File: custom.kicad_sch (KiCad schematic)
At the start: 43 parts, among them J1 OLED_128x32, SW1 Switch, U1 Nice_Nano_V2

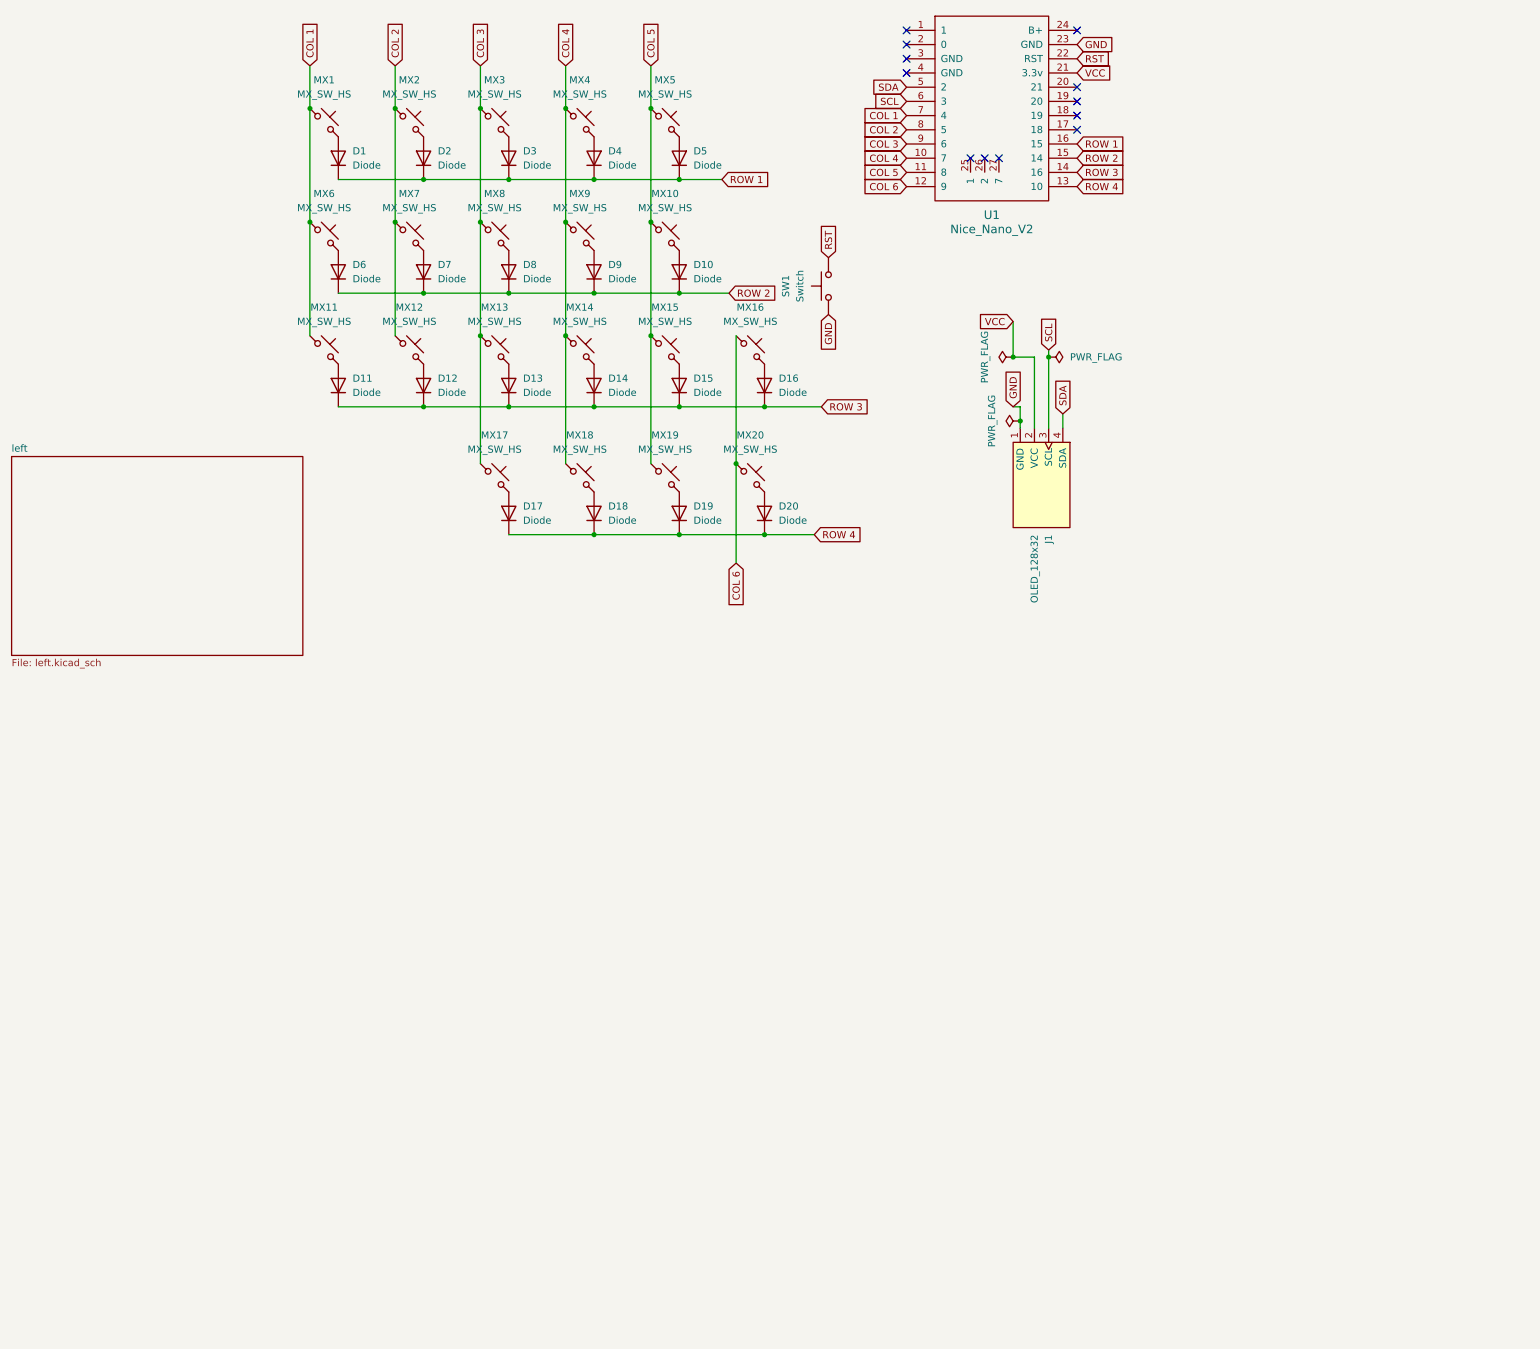
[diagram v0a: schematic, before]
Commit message: Formato de teclado listo
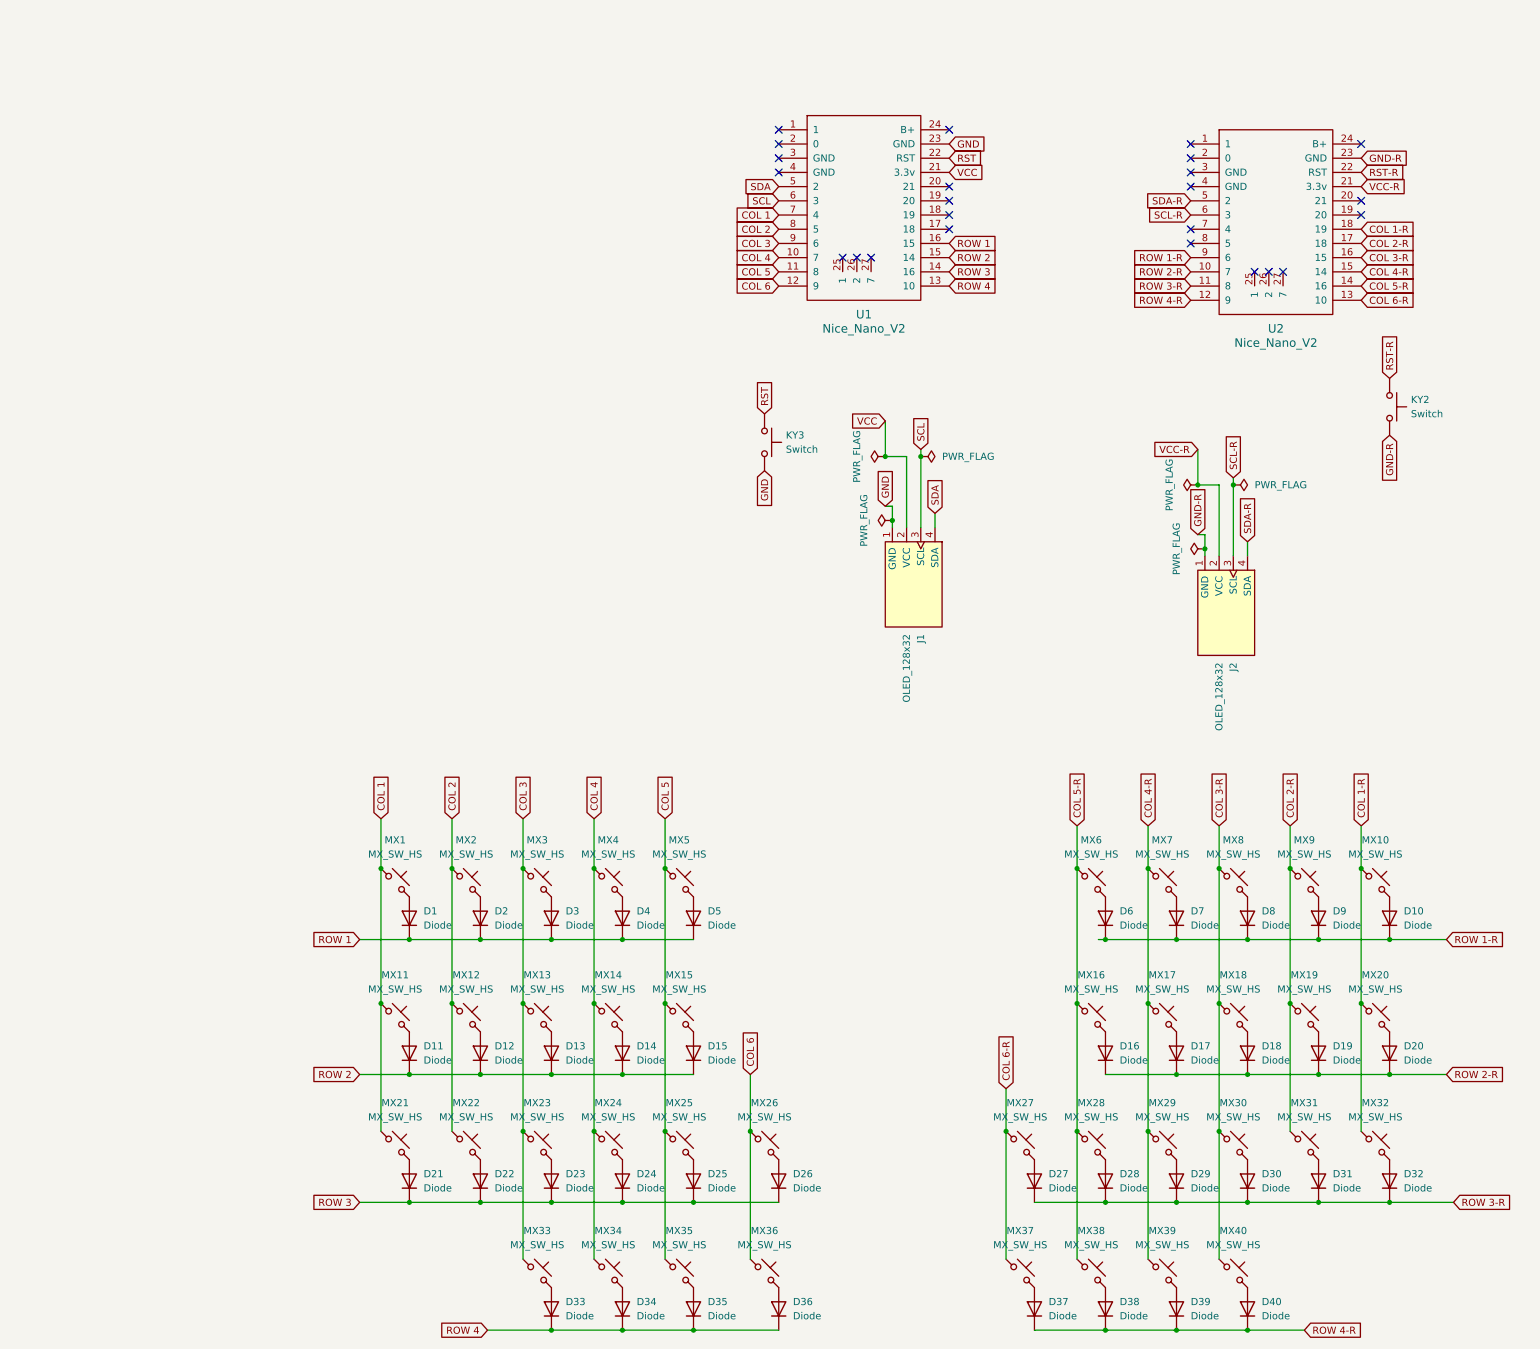
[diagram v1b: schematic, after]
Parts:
- removed SW1: Switch, Button_Switch_SMD:SW_Push_1P1T_NO_Vertical_Wuerth_434133025816, symbol ScottoKeebs:Placeholder_Switch
- added D21, D22, D23, D24, D25, D26, D27, D28, D29, D30, D31, D32, D33, D34, D35, D36, D37, D38, D39, D40: Diode, symbol ScottoKeebs:Placeholder_Diode
- added J2: OLED_128x32, ScottoKeebs_Components:OLED_128x32, symbol ScottoKeebs:OLED_128x32
- added KY2, KY3: Switch, Button_Switch_SMD:SW_Push_1P1T_NO_Vertical_Wuerth_434133025816, symbol ScottoKeebs:Placeholder_Switch
- added MX21, MX22, MX23, MX24, MX25, MX26, MX27, MX28, MX29, MX30, MX31, MX32, MX33, MX34, MX35, MX38, MX39, MX40: MX_SW_HS, PCM_marbastlib-mx:SW_MX_HS_CPG151101S11_1u, symbol PCM_marbastlib-mx:MX_SW_HS_CPG151101S11
- added MX36, MX37: MX_SW_HS, PCM_marbastlib-mx:SW_MX_HS_CPG151101S11_1.25u, symbol PCM_marbastlib-mx:MX_SW_HS_CPG151101S11
- added U2: Nice_Nano_V2, ScottoKeebs_MCU:Nice_Nano_V2, symbol ScottoKeebs:MCU_Nice_Nano_V2
- D1, D10, D11, D12, D13, D14, D15, D16, D17, D18, D19, D2, D20, D3, D4, D5, D6, D7, D8, D9: footprint Diode_SMD:D_SOD-123 -> (none)
- MX20: footprint PCM_marbastlib-mx:SW_MX_HS_CPG151101S11_1.25u -> PCM_marbastlib-mx:SW_MX_HS_CPG151101S11_1u
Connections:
- net COL 1: now also MX21.1; no longer MX6.1
- net COL 2: now also MX22.1; no longer MX7.1
- net COL 3: now also MX23.1, MX33.1; no longer MX17.1, MX8.1
- net COL 4: now also MX24.1, MX34.1; no longer MX18.1, MX9.1
- net COL 5: now also MX25.1, MX35.1; no longer MX10.1, MX19.1
- net COL 6: now also MX26.1, MX36.1; no longer MX16.1, MX20.1
- net GND: now also KY3.1
- net ROW 2: now also D11.1 (K), D12.1 (K), D13.1 (K), D14.1 (K), D15.1 (K); no longer D10.1 (K), D6.1 (K), D7.1 (K), D8.1 (K), D9.1 (K)
- net ROW 3: now also D21.1 (K), D22.1 (K), D23.1 (K), D24.1 (K), D25.1 (K), D26.1 (K); no longer D11.1 (K), D12.1 (K), D13.1 (K), D14.1 (K), D15.1 (K), D16.1 (K)
- net ROW 4: now also D33.1 (K), D34.1 (K), D35.1 (K), D36.1 (K); no longer D17.1 (K), D18.1 (K), D19.1 (K), D20.1 (K)
- net RST: now also KY3.2
- new net: D35.2 (A), MX35.2
- new net: D29.2 (A), MX29.2
- new net: D21.2 (A), MX21.2
- new net: D24.2 (A), MX24.2
- new net: D38.2 (A), MX38.2
- new net: D28.2 (A), MX28.2
- new net: D22.2 (A), MX22.2
- new net: D30.2 (A), MX30.2
- new net: D27.2 (A), MX27.2
- new net: D26.2 (A), MX26.2
- new net: D23.2 (A), MX23.2
- new net: D39.2 (A), MX39.2
- new net: D34.2 (A), MX34.2
- new net: D31.2 (A), MX31.2
- new net: D25.2 (A), MX25.2
- new net: D36.2 (A), MX36.2
- new net: D40.2 (A), MX40.2
- new net: D33.2 (A), MX33.2
- new net: D32.2 (A), MX32.2
- new net: D37.2 (A), MX37.2
- new net COL 1-R: MX10.1, MX20.1, MX32.1, U2.18 (19)
- new net COL 2-R: MX19.1, MX31.1, MX9.1, U2.17 (18)
- new net COL 3-R: MX18.1, MX30.1, MX40.1, MX8.1, U2.16 (15)
- new net COL 4-R: MX17.1, MX29.1, MX39.1, MX7.1, U2.15 (14)
- new net COL 5-R: MX16.1, MX28.1, MX38.1, MX6.1, U2.14 (16)
- new net COL 6-R: MX27.1, MX37.1, U2.13 (10)
- new net GND-R: J2.1 (GND), KY2.1, U2.23 (GND)
- new net ROW 1-R: D10.1 (K), D6.1 (K), D7.1 (K), D8.1 (K), D9.1 (K), U2.9 (6)
- new net ROW 2-R: D16.1 (K), D17.1 (K), D18.1 (K), D19.1 (K), D20.1 (K), U2.10 (7)
- new net ROW 3-R: D27.1 (K), D28.1 (K), D29.1 (K), D30.1 (K), D31.1 (K), D32.1 (K), U2.11 (8)
- new net ROW 4-R: D37.1 (K), D38.1 (K), D39.1 (K), D40.1 (K), U2.12 (9)
- new net RST-R: KY2.2, U2.22 (RST)
- new net SCL-R: J2.3 (SCL), U2.6 (3)
- new net SDA-R: J2.4 (SDA), U2.5 (2)
- new net VCC-R: J2.2 (VCC), U2.21 (3.3v)
- no-connect marks 12 -> 24
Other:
- removed sheet left
- moved on the sheet: J1, U1
